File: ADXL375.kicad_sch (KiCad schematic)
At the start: 5 parts, among them U9 ADXL372BCCZ-RL

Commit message: C14 y C1,C2,... modificados
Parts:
- C36, C37: LCSC Part C5448844 -> C282518
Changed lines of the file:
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@@
 			)
 		)
-		(property "Datasheet" "https://www.lcsc.com/datasheet/C5448844.pdf"
+		(property "Datasheet" "https://www.lcsc.com/datasheet/C282518.pdf?spm=wm.sxq.inf.ggs___wm.fly.bg.0.cbh&lcsc_vid=FVBZXlJVElFWAVdTTgAPVAcHR1hXAlIFT1cMUAFWQVYxVlNeRFBfVlJeQ1VXXzsOAxUeFF5JWBYZEEoKFBINSQcJGk4NBhADEA4cHktXRlVcSQwSGg0%3D"
 			(at 138.43 96.52 0)
 			(hide yes)
@@
 			)
 		)
-		(property "LCSC Part" "C5448844"
+		(property "LCSC Part" "C282518"
 			(at 146.05 96.52 0)
+			(hide yes)
+			(show_name no)
+			(do_not_autoplace no)
+			(effects
+				(font
+					(size 1.27 1.27)
+				)
+			)
+		)
+		(property "Field7" ""
+			(at 128.27 96.52 90)
 			(hide yes)
 			(show_name no)
@@
 			)
 		)
-		(property "Datasheet" "https://www.lcsc.com/datasheet/C5448844.pdf"
+		(property "Datasheet" "https://www.lcsc.com/datasheet/C282518.pdf?spm=wm.sxq.inf.ggs___wm.fly.bg.0.cbh&lcsc_vid=FVBZXlJVElFWAVdTTgAPVAcHR1hXAlIFT1cMUAFWQVYxVlNeRFBfVlJeQ1VXXzsOAxUeFF5JWBYZEEoKFBINSQcJGk4NBhADEA4cHktXRlVcSQwSGg0%3D"
 			(at 215.9 101.6 0)
 			(hide yes)
@@
 			)
 		)
-		(property "LCSC Part" "C5448844"
+		(property "LCSC Part" "C282518"
 			(at 223.52 101.6 0)
+			(hide yes)
+			(show_name no)
+			(do_not_autoplace no)
+			(effects
+				(font
+					(size 1.27 1.27)
+				)
+			)
+		)
+		(property "Field7" ""
+			(at 205.74 101.6 90)
 			(hide yes)
 			(show_name no)
@@
 			)
 		)
+		(property "Field7" ""
+			(at 171.45 97.79 0)
+			(hide yes)
+			(show_name no)
+			(do_not_autoplace no)
+			(effects
+				(font
+					(size 1.27 1.27)
+				)
+			)
+		)
 		(pin "10"
 		)
@@
 			)
 		)
+		(property "Field7" ""
+			(at 228.6 93.98 0)
+			(hide yes)
+			(show_name no)
+			(do_not_autoplace no)
+			(effects
+				(font
+					(size 1.27 1.27)
+				)
+			)
+		)
 		(pin "2"
 		)
@@
 			(hide yes)
 			(show_name no)
+			(do_not_autoplace no)
+			(effects
+				(font
+					(size 1.27 1.27)
+				)
+			)
+		)
+		(property "Field7" ""
+			(at 218.44 101.6 90)
+			(hide yes)
+			(show_name no)

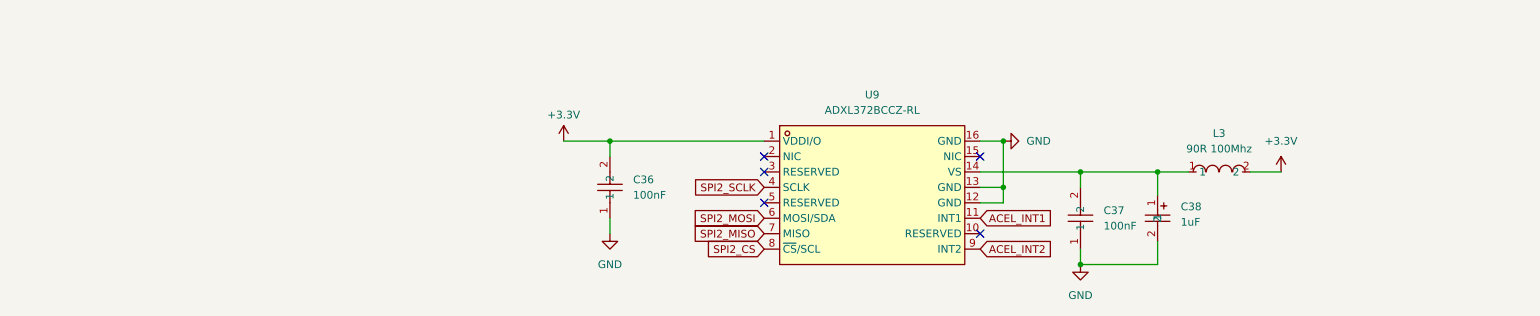
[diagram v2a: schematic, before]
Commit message: Avance 02/08
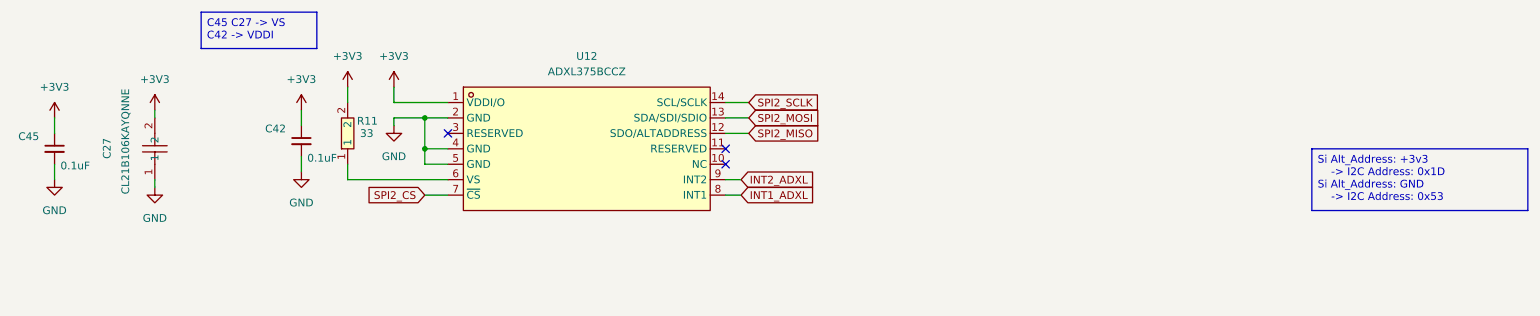
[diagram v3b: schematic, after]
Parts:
- removed C36, C37: 100nF, Capacitor_SMD:C_0603_1608Metric_Pad1.08x0.95mm_HandSolder, symbol CANSAT_STM32_symbols:TCC0402X7R104J500AT
- removed C38: 1uF, ARLISS-footprints:CAP-SMD_L3.5-W2.8-R-RD, symbol CANSAT_STM32_symbols:TAJB105K035RNJ
- removed L3: 90R 100Mhz, Inductor_SMD:L_0603_1608Metric_Pad1.05x0.95mm_HandSolder, symbol CANSAT_STM32_symbols:CBG100505U000T
- removed U9: ADXL372BCCZ-RL, ARLISS-footprints:LGA-16_L3.3-W3.0-P0.50-TL, symbol CANSAT_STM32_symbols:ADXL372BCCZ-RL
- added C27: CL21B106KAYQNNE, easyeda2kicad:C0805, symbol CANSAT_STM32_symbols:CL21B106KAYQNNE
- added C42, C45: 0.1uF, Capacitor_SMD:C_0603_1608Metric, symbol Device:C_Small
- added R11: 33, Resistor_SMD:R_0603_1608Metric_Pad0.98x0.95mm_HandSolder, symbol CANSAT_STM32_symbols:RC0603FR-074K7L
- added U12: ADXL375BCCZ, ARLISS-footprints:LGA-14_L5.0-W3.0-P0.80-BL, symbol easyeda2kicad:ADXL375BCCZ
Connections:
- net GND: now also C27.1, C42.2, C45.2, U12.2 (GND), U12.4 (GND), U12.5 (GND)
- net SPI2_CS: now also U12.7 (~{CS})
- net SPI2_MISO: now also U12.12 (SDO/ALTADDRESS)
- net SPI2_MOSI: now also U12.13 (SDA/SDI/SDIO)
- net SPI2_SCLK: now also U12.14 (SCL/SCLK)
- new net: R11.1, U12.6 (VS)
- new net +3V3: C27.2, C42.1, C45.1, R11.2, U12.1 (VDDI/O)
- new net INT1_ADXL: U12.8 (INT1)
- new net INT2_ADXL: U12.9 (INT2)
- no-connect marks 5 -> 3
